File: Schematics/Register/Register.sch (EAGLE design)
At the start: 42 parts

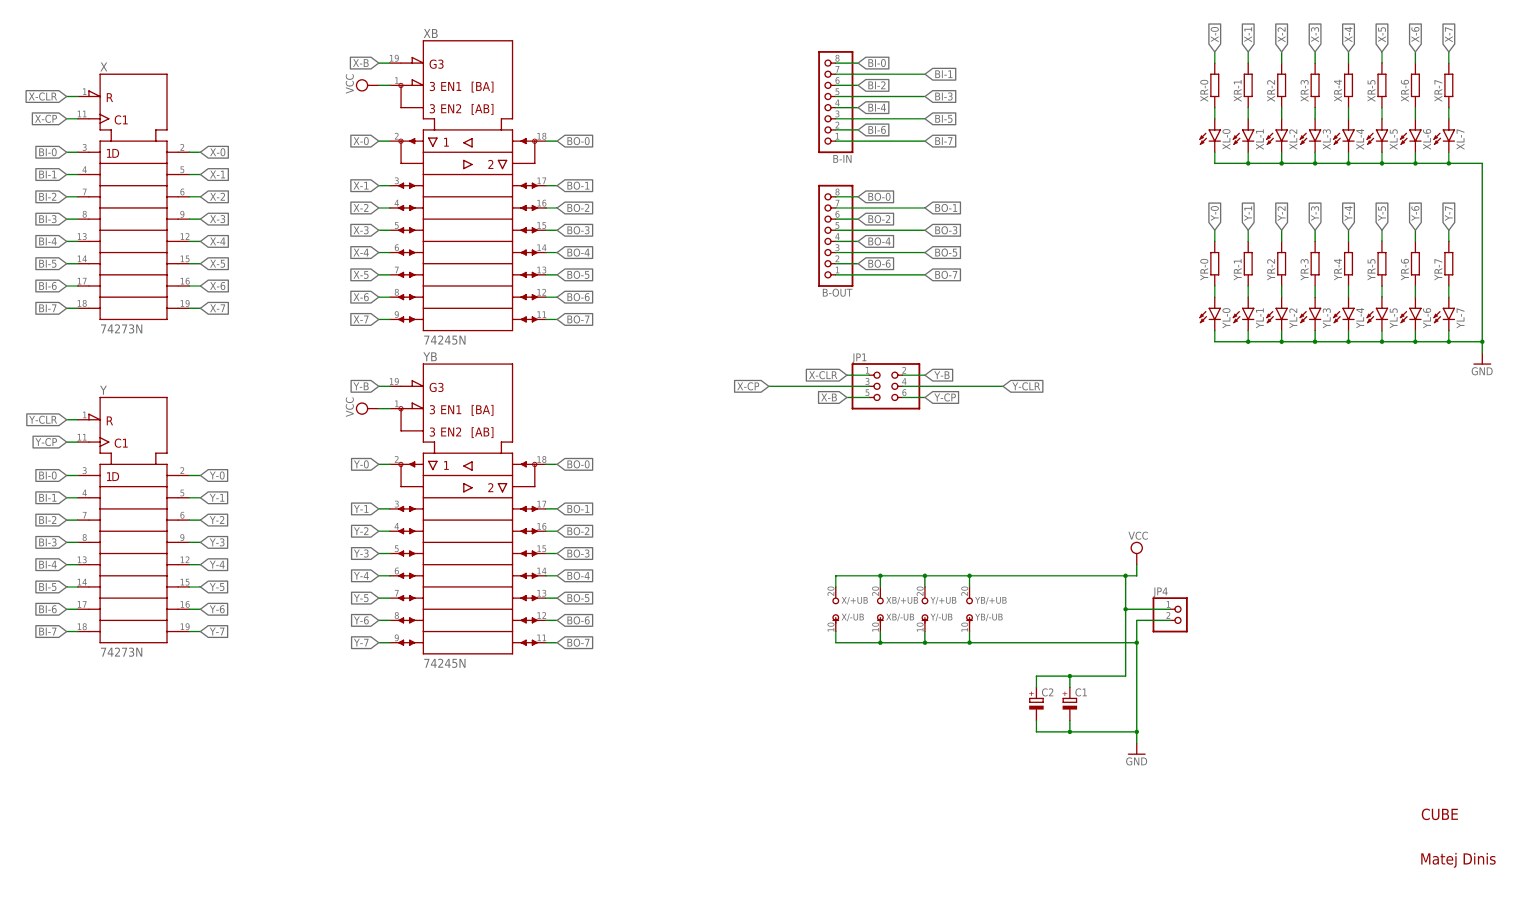
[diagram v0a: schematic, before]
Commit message: Added register.
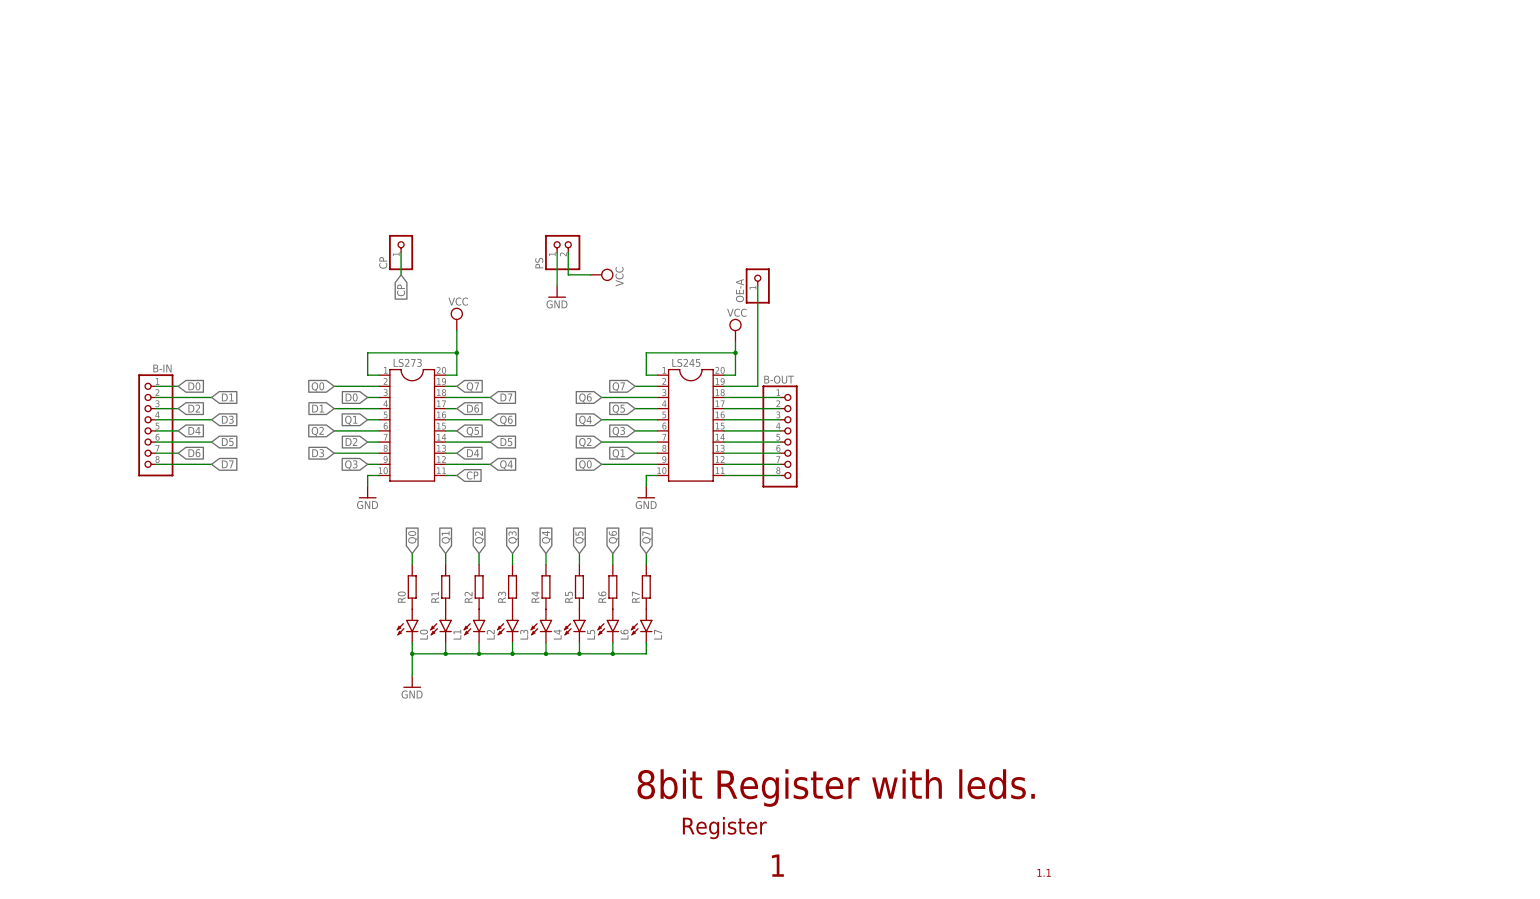
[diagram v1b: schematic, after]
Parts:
- removed C1, C2: (no value), rcl:CPOL-EUE3.5-8
- removed JP1: (no value), pinhead:PINHD-2X3
- removed JP4: (no value), pinhead:PINHD-1X2
- removed X, Y: 74273N, 74ttl-din:74273N
- removed XB, YB: 74245N, 74ttl-din:74245N
- removed XL-0, XL-1, XL-2, XL-3, XL-4, XL-5, XL-6, XL-7, YL-0, YL-1, YL-2, YL-3, YL-4, YL-5, YL-6, YL-7: (no value), led:LED5MM
- removed XR-0, XR-1, XR-2, XR-3, XR-4, XR-5, XR-6, XR-7, YR-0, YR-1, YR-2, YR-3, YR-4, YR-5, YR-6, YR-7: (no value), rcl:R-EU_0207/10
- added CP, OE-A: (no value), pinhead:PINHD-1X1
- added L0, L1, L2, L3, L4, L5, L6, L7: (no value), led:LED5MM
- added LS245, LS273: (no value), ic-package:DIL20S
- added PS: (no value), pinhead:PINHD-1X2
- added R0, R1, R2, R3, R4, R5, R6, R7: (no value), rcl:R-EU_0204/7
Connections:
- removed net BI-0: B-IN.8, X1.1D, Y1.1D
- removed net BI-1: B-IN.7, X1.2D, Y1.2D
- removed net BI-2: B-IN.6, X1.3D, Y1.3D
- removed net BI-3: B-IN.5, X1.4D, Y1.4D
- removed net BI-4: B-IN.4, X1.5D, Y1.5D
- removed net BI-5: B-IN.3, X1.6D, Y1.6D
- removed net BI-6: B-IN.2, X1.7D, Y1.7D
- removed net BI-7: B-IN.1, X1.8D, Y1.8D
- removed net BO-0: B-OUT.8, XB1.B1, YB1.B1
- removed net BO-1: B-OUT.7, XB1.B2, YB1.B2
- removed net BO-2: B-OUT.6, XB1.B3, YB1.B3
- removed net BO-3: B-OUT.5, XB1.B4, YB1.B4
- removed net BO-4: B-OUT.4, XB1.B5, YB1.B5
- removed net BO-5: B-OUT.3, XB1.B6, YB1.B6
- removed net BO-6: B-OUT.2, XB1.B7, YB1.B7
- removed net BO-7: B-OUT.1, XB1.B8, YB1.B8
- removed net N$113: XL-1.A, XR-1.1
- removed net N$116: XL-2.A, XR-2.1
- removed net N$119: XL-3.A, XR-3.1
- removed net N$122: XL-4.A, XR-4.1
- removed net N$125: XL-5.A, XR-5.1
- removed net N$128: XL-6.A, XR-6.1
- removed net N$131: XL-7.A, XR-7.1
- removed net N$134: YL-0.A, YR-0.1
- removed net N$137: YL-1.A, YR-1.1
- removed net N$140: YL-2.A, YR-2.1
- removed net N$143: YL-3.A, YR-3.1
- removed net N$146: YL-4.A, YR-4.1
- removed net N$149: YL-5.A, YR-5.1
- removed net N$152: YL-6.A, YR-6.1
- removed net N$155: YL-7.A, YR-7.1
- removed net N$2: XL-0.A, XR-0.1
- removed net X-0: X1.1Q, XB1.A1, XR-0.2
- removed net X-1: X1.2Q, XB1.A2, XR-1.2
- removed net X-2: X1.3Q, XB1.A3, XR-2.2
- removed net X-3: X1.4Q, XB1.A4, XR-3.2
- removed net X-4: X1.5Q, XB1.A5, XR-4.2
- removed net X-5: X1.6Q, XB1.A6, XR-5.2
- removed net X-6: X1.7Q, XB1.A7, XR-6.2
- removed net X-7: X1.8Q, XB1.A8, XR-7.2
- removed net X-B: JP1.5, XB1.!G
- removed net X-CLR: JP1.1, X1.!CLR
- removed net X-CP: JP1.3, X1.CLK
- removed net Y-0: Y1.1Q, YB1.A1, YR-0.2
- removed net Y-1: Y1.2Q, YB1.A2, YR-1.2
- removed net Y-2: Y1.3Q, YB1.A3, YR-2.2
- removed net Y-3: Y1.4Q, YB1.A4, YR-3.2
- removed net Y-4: Y1.5Q, YB1.A5, YR-4.2
- removed net Y-5: Y1.6Q, YB1.A6, YR-5.2
- removed net Y-6: Y1.7Q, YB1.A7, YR-6.2
- removed net Y-7: Y1.8Q, YB1.A8, YR-7.2
- removed net Y-B: JP1.2, YB1.!G
- removed net Y-CLR: JP1.4, Y1.!CLR
- removed net Y-CP: JP1.6, Y1.CLK
- new net BO0: B-OUT.8, LS245.11
- new net BO1: B-OUT.7, LS245.12
- new net BO2: B-OUT.6, LS245.13
- new net BO3: B-OUT.5, LS245.14
- new net BO4: B-OUT.4, LS245.15
- new net BO5: B-OUT.3, LS245.16
- new net BO6: B-OUT.2, LS245.17
- new net BO7: B-OUT.1, LS245.18
- new net CP: CP.1, LS273.11
- new net D0: B-IN.1, LS273.3
- new net D1: B-IN.2, LS273.4
- new net D2: B-IN.3, LS273.7
- new net D3: B-IN.4, LS273.8
- new net D4: B-IN.5, LS273.13
- new net D5: B-IN.6, LS273.14
- new net D6: B-IN.7, LS273.17
- new net D7: B-IN.8, LS273.18
- new net N$1: L7.A, R7.1
- new net N$10: L1.A, R1.1
- new net N$11: L0.A, R0.1
- new net N$18: LS245.19, OE-A.1
- new net N$5: L6.A, R6.1
- new net N$6: L5.A, R5.1
- new net N$7: L4.A, R4.1
- new net N$8: L3.A, R3.1
- new net N$9: L2.A, R2.1
- new net Q0: LS245.9, LS273.2, R0.2
- new net Q1: LS245.8, LS273.5, R1.2
- new net Q2: LS245.7, LS273.6, R2.2
- new net Q3: LS245.6, LS273.9, R3.2
- new net Q4: LS245.5, LS273.12, R4.2
- new net Q5: LS245.4, LS273.15, R5.2
- new net Q6: LS245.3, LS273.16, R6.2
- new net Q7: LS245.2, LS273.19, R7.2
- net GND: now also L0.C, L1.C, L2.C, L3.C, L4.C, L5.C, L6.C, L7.C, LS245.10, LS273.10, PS.1; no longer C1.-, C2.-, JP4.2, X/-UB.-UB, XB/-UB.-UB, XL-0.C, XL-1.C, XL-2.C, XL-3.C, XL-4.C, XL-5.C, XL-6.C, XL-7.C, Y/-UB.-UB, YB/-UB.-UB, YL-0.C, YL-1.C, YL-2.C, YL-3.C, YL-4.C, YL-5.C, YL-6.C, YL-7.C
- net VCC: now also LS245.1, LS245.20, LS273.1, LS273.20, PS.2; no longer C1.+, C2.+, JP4.1, X/+UB.+UB, XB/+UB.+UB, XB1.DIR, Y/+UB.+UB, YB/+UB.+UB, YB1.DIR
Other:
- note added: "1"
- note added: "1.1"
- note added: "8bit Register with leds."
- note added: "Register"
- note removed: "CUBE"
- note removed: "Matej Dinis"
- moved on the sheet: B-IN, B-OUT
